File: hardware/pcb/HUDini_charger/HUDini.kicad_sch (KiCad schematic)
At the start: 21 parts, among them J2 Conn_01x06_Pin, J3 Conn_01x06_Pin, J4 Conn_01x07_Pin, SW1 RESET, SW3 PWR_REC, U5 MDBT42Q-512K

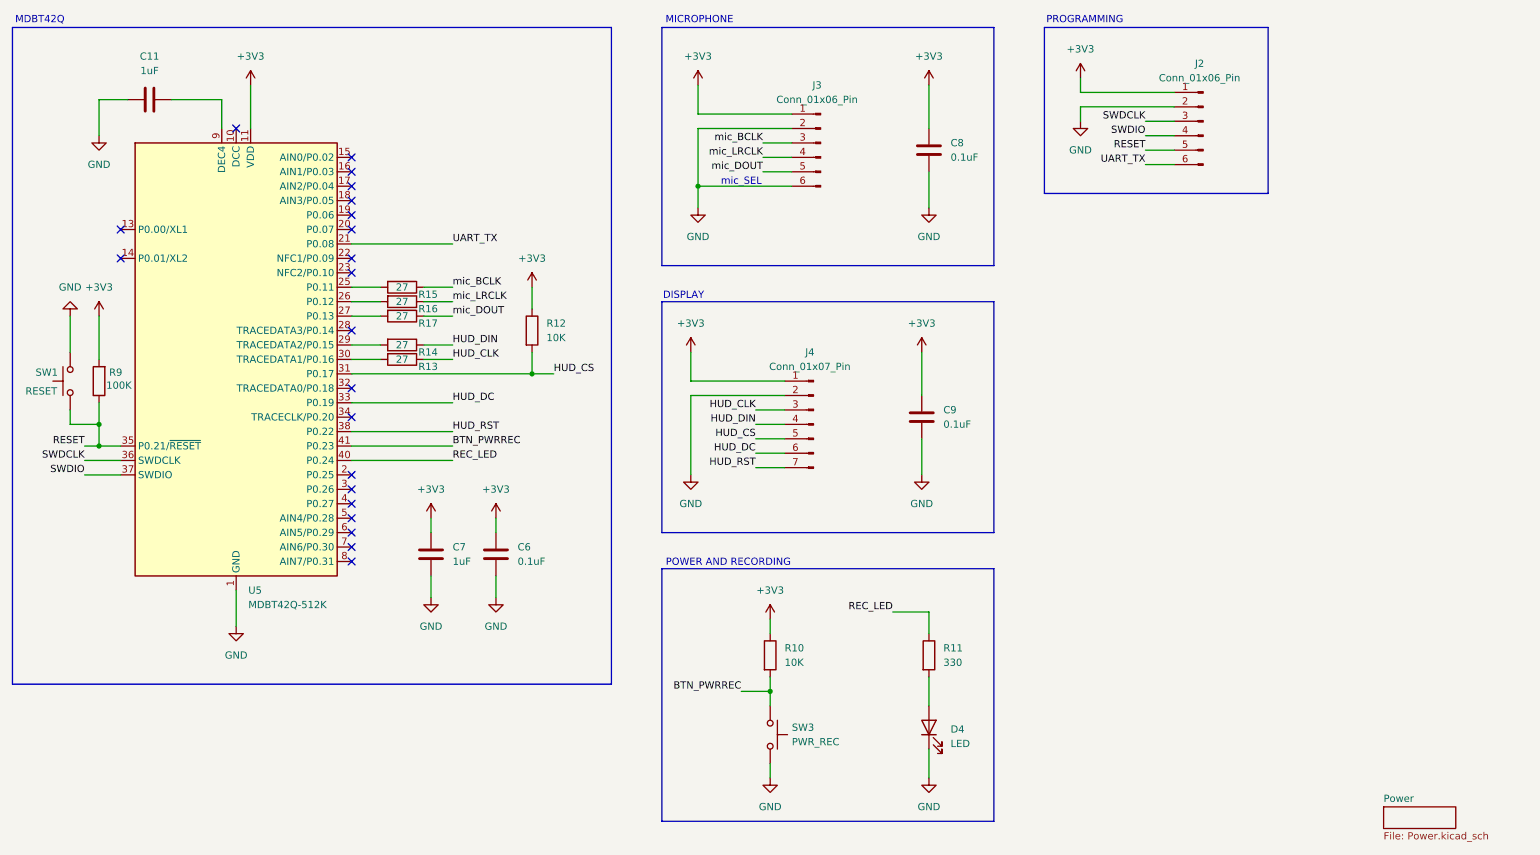
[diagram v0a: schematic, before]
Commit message: Updated PCB Files
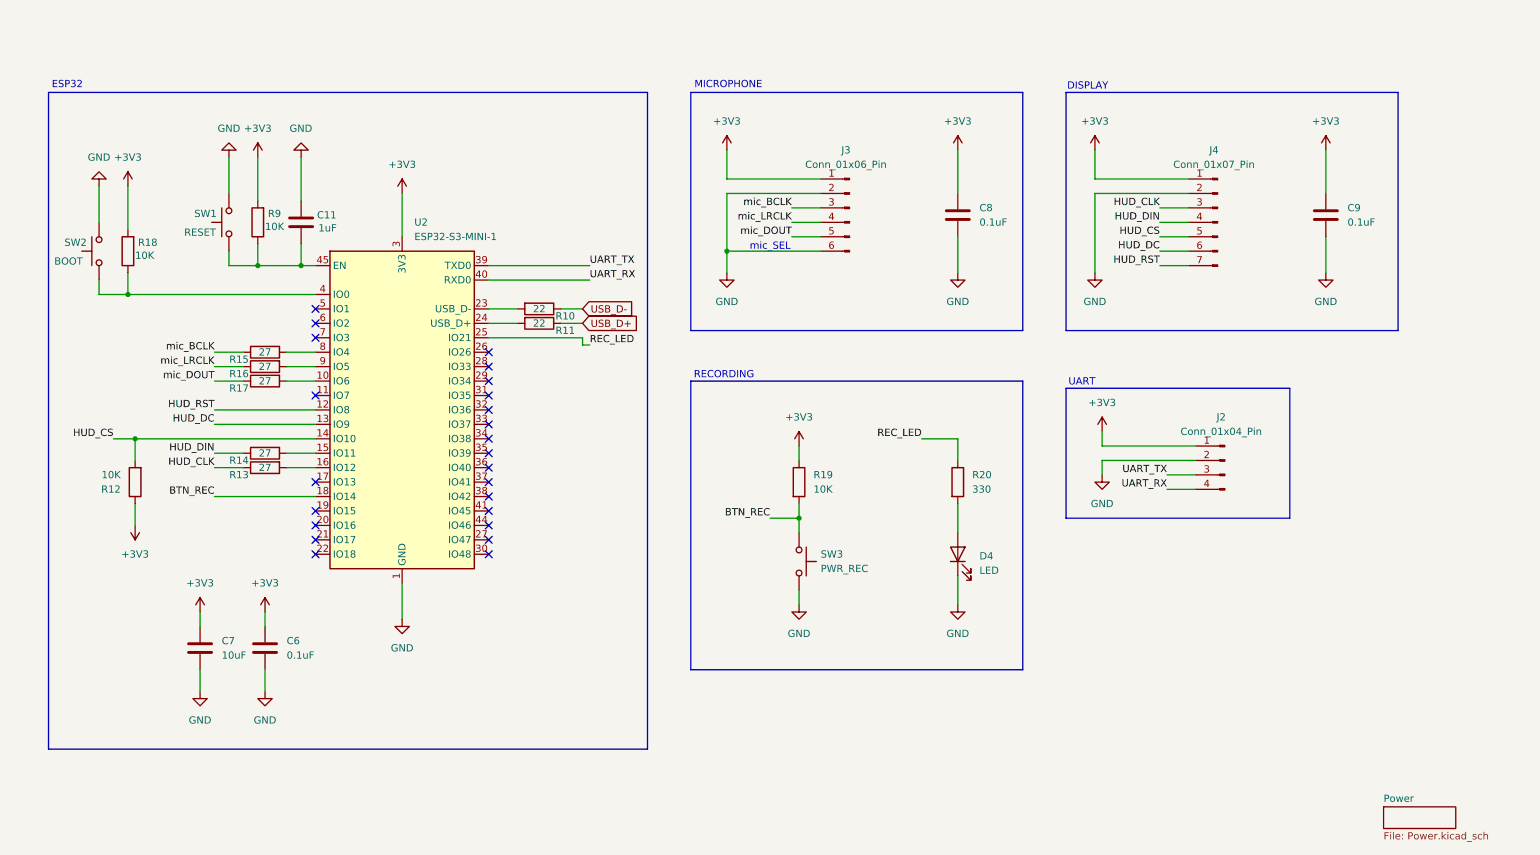
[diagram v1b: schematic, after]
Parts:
- removed J2: Conn_01x06_Pin, Connector_PinHeader_2.54mm:PinHeader_1x06_P2.54mm_Vertical, symbol Connector:Conn_01x06_Pin
- removed U5: MDBT42Q-512K, RF_Module:Raytac_MDBT42Q, symbol RF_Module:MDBT42Q-512K
- added J2: Conn_01x04_Pin, Connector_Wire:SolderWire-0.15sqmm_1x04_P4mm_D0.5mm_OD1.5mm, symbol Connector:Conn_01x04_Pin
- added R10, R11: 22, Resistor_SMD:R_0603_1608Metric_Pad0.98x0.95mm_HandSolder, symbol Device:R
- added R18: 10K, Resistor_SMD:R_0603_1608Metric_Pad0.98x0.95mm_HandSolder, symbol Device:R
- added SW2: BOOT, Button_Switch_SMD:SW_SPST_PTS810, symbol Switch:SW_Push
- added U2: ESP32-S3-MINI-1, RF_Module:ESP32-S2-MINI-1, symbol RF_Module:ESP32-S3-MINI-1
- C11, C6, C9: footprint Capacitor_SMD:C_0603_1608Metric -> Capacitor_SMD:C_0603_1608Metric_Pad1.08x0.95mm_HandSolder
- C7: value 1uF -> 10uF; footprint Capacitor_SMD:C_0603_1608Metric -> Capacitor_SMD:C_0603_1608Metric_Pad1.08x0.95mm_HandSolder
- D4: footprint LED_SMD:LED_0603_1608Metric -> LED_SMD:LED_0603_1608Metric_Pad1.05x0.95mm_HandSolder
- J3: footprint Connector_PinHeader_2.54mm:PinHeader_1x06_P2.54mm_Vertical -> Connector_Wire:SolderWire-0.15sqmm_1x06_P4mm_D0.5mm_OD1.5mm
- J4: footprint Connector_PinHeader_2.54mm:PinHeader_1x07_P2.54mm_Horizontal -> Connector_PinHeader_1.00mm:PinHeader_1x07_P1.00mm_Horizontal
- R12, R13, R14, R15, R16, R17: footprint Resistor_SMD:R_0603_1608Metric -> Resistor_SMD:R_0603_1608Metric_Pad0.98x0.95mm_HandSolder
- R19: renamed from R10; footprint Resistor_SMD:R_0603_1608Metric -> Resistor_SMD:R_0603_1608Metric_Pad0.98x0.95mm_HandSolder
- R20: renamed from R11; footprint Resistor_SMD:R_0603_1608Metric -> Resistor_SMD:R_0603_1608Metric_Pad0.98x0.95mm_HandSolder
- R9: value 100K -> 10K; footprint Resistor_SMD:R_0603_1608Metric -> Resistor_SMD:R_0603_1608Metric_Pad0.98x0.95mm_HandSolder
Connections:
- net +3V3: now also J2.1 (Pin_1), R18.2, U2.3 (3V3)
- net GND: now also C11.2, J2.2 (Pin_2), SW2.2, U2.1 (GND), U2.2 (GND), U2.42 (GND), U2.43 (GND), U2.46 (GND), U2.47 (GND), U2.48 (GND), U2.49 (GND), U2.50 (GND), U2.51 (GND), U2.52 (GND), U2.53 (GND), U2.54 (GND), U2.55 (GND), U2.56 (GND), U2.57 (GND), U2.58 (GND), U2.59 (GND), U2.60 (GND), U2.61 (GND), U2.62 (GND), U2.63 (GND), U2.64 (GND), U2.65 (GND); no longer C11.1
- net HUD_CS: now also U2.14 (IO10)
- net HUD_DC: now also U2.13 (IO9)
- net HUD_RST: now also U2.12 (IO8)
- net REC_LED: now also U2.25 (IO21)
- net UART_TX: now also J2.3 (Pin_3), U2.39 (TXD0)
- net at R14.2: now also U2.15 (IO11)
- net at R16.2: now also U2.9 (IO5)
- net at R15.2: now also U2.8 (IO4)
- net at R17.2: now also U2.10 (IO6)
- net at R13.2: now also U2.16 (IO12)
- net BTN_PWRREC renamed BTN_REC
- net BTN_REC: now also U2.18 (IO14)
- net RESET: no longer names the net of R9.1, SW1.1
- net RESET: now also C11.1, U2.45 (EN)
- new net: R18.1, SW2.1, U2.4 (IO0)
- new net: R11.2, U2.24 (USB_D+)
- new net: R10.2, U2.23 (USB_D-)
- new net UART_RX: J2.4 (Pin_4), U2.40 (RXD0)
- new net USB_D+: R11.1
- new net USB_D-: R10.1
- no-connect marks 21 -> 24
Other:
- note added: "ESP32"
- note added: "RECORDING"
- note added: "UART"
- note removed: "MDBT42Q"
- note removed: "POWER AND RECORDING"
- note removed: "PROGRAMMING"
- moved on the sheet: C11, C6, C7, C8, C9, D4, J3, J4, R12, R13, R14, R15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

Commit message: More Progress
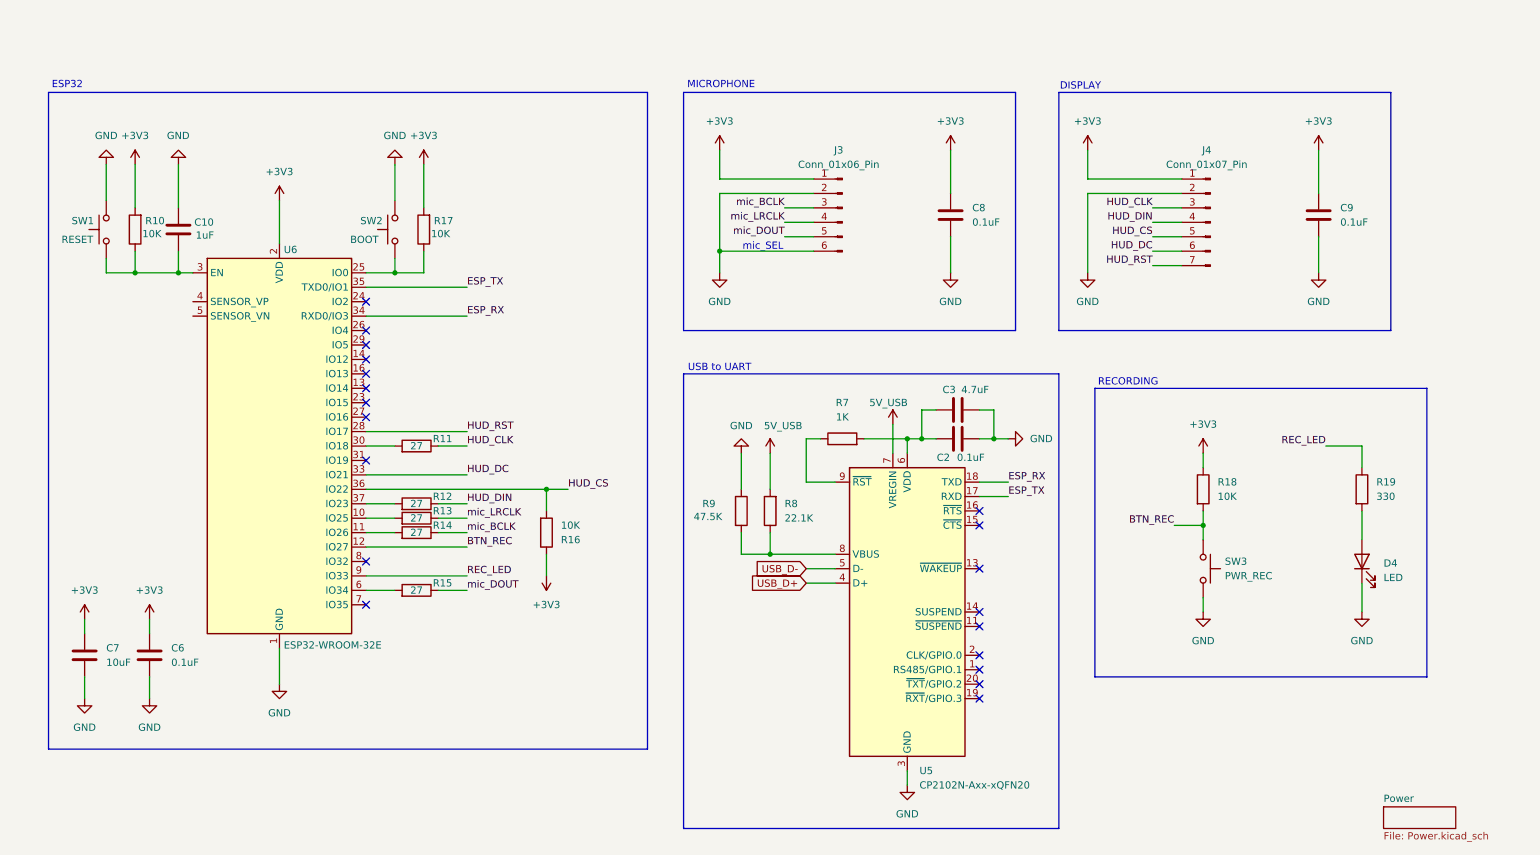
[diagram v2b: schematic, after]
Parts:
- removed J2: Conn_01x04_Pin, Connector_Wire:SolderWire-0.15sqmm_1x04_P4mm_D0.5mm_OD1.5mm, symbol Connector:Conn_01x04_Pin
- removed R10, R11: 22, Resistor_SMD:R_0603_1608Metric_Pad0.98x0.95mm_HandSolder, symbol Device:R
- removed U2: ESP32-S3-MINI-1, RF_Module:ESP32-S2-MINI-1, symbol RF_Module:ESP32-S3-MINI-1
- added C2: 0.1uF, Capacitor_SMD:C_0603_1608Metric_Pad1.08x0.95mm_HandSolder, symbol Device:C
- added C3: 4.7uF, Capacitor_SMD:C_0603_1608Metric_Pad1.08x0.95mm_HandSolder, symbol Device:C
- added R7: 1K, Resistor_SMD:R_0603_1608Metric_Pad0.98x0.95mm_HandSolder, symbol Device:R
- added R8: 22.1K, Resistor_SMD:R_0603_1608Metric_Pad0.98x0.95mm_HandSolder, symbol Device:R
- added R9: 47.5K, Resistor_SMD:R_0603_1608Metric_Pad0.98x0.95mm_HandSolder, symbol Device:R
- added U5: CP2102N-Axx-xQFN20, Package_DFN_QFN:SiliconLabs_QFN-20-1EP_3x3mm_P0.5mm_EP1.8x1.8mm, symbol Interface_USB:CP2102N-Axx-xQFN20
- added U6: ESP32-WROOM-32E, RF_Module:ESP32-WROOM-32D, symbol RF_Module:ESP32-WROOM-32E
- renumbered C11 to C10, R9 to R10, R13 to R11, R14 to R12, R16 to R13, R15 to R14, R17 to R15, R12 to R16, R18 to R17, R19 to R18, R20 to R19
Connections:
- net +3V3: now also U6.2 (VDD)
- net BTN_REC: now also U6.12 (IO27)
- net GND: now also C2.2, C3.2, R9.1, U5.12 (GND), U5.21 (GND), U5.3 (GND), U6.1 (GND), U6.15 (GND), U6.38 (GND), U6.39 (GND)
- net HUD_CS: now also U6.36 (IO22)
- net HUD_DC: now also U6.33 (IO21)
- net HUD_RST: now also U6.28 (IO17)
- net REC_LED: now also U6.9 (IO33)
- net USB_D+: now also U5.4 (D+)
- net USB_D-: now also U5.5 (D-)
- net at R17.1, SW2.1: now also U6.25 (IO0)
- net at C10.1, R10.1, SW1.1: now also U6.3 (EN)
- net at R12.2: now also U6.37 (IO23)
- net at R13.2: now also U6.10 (IO25)
- net at R14.2: now also U6.11 (IO26)
- net at R15.2: now also U6.6 (IO34)
- net at R11.2: now also U6.30 (IO18)
- new net: C2.1, C3.1, R7.2, U5.6 (VDD)
- new net: R8.1, R9.2, U5.8 (VBUS)
- new net: R7.1, U5.9 (~{RST})
- new net 5V_USB: R8.2, U5.7 (VREGIN)
- new net ESP_RX: U5.18 (TXD), U6.34 (RXD0/IO3)
- new net ESP_TX: U5.17 (RXD), U6.35 (TXD0/IO1)
- no-connect marks 24 -> 20
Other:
- note added: "USB to UART"
- note removed: "UART"
- moved on the sheet: C10, C6, C7, C8, C9, D4, J3, J4, R10, R11, R12, R13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
